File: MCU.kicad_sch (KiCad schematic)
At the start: 44 parts, among them J1 *, J3 *, J4 *, U1 *

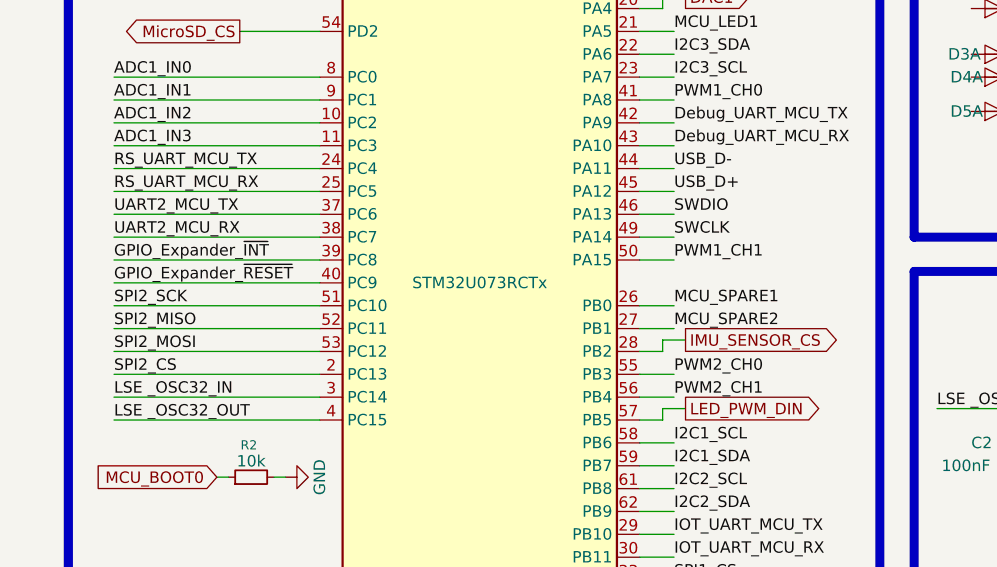
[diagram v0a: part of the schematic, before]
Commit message: [Schematic][Add] MCU Expander Schematic
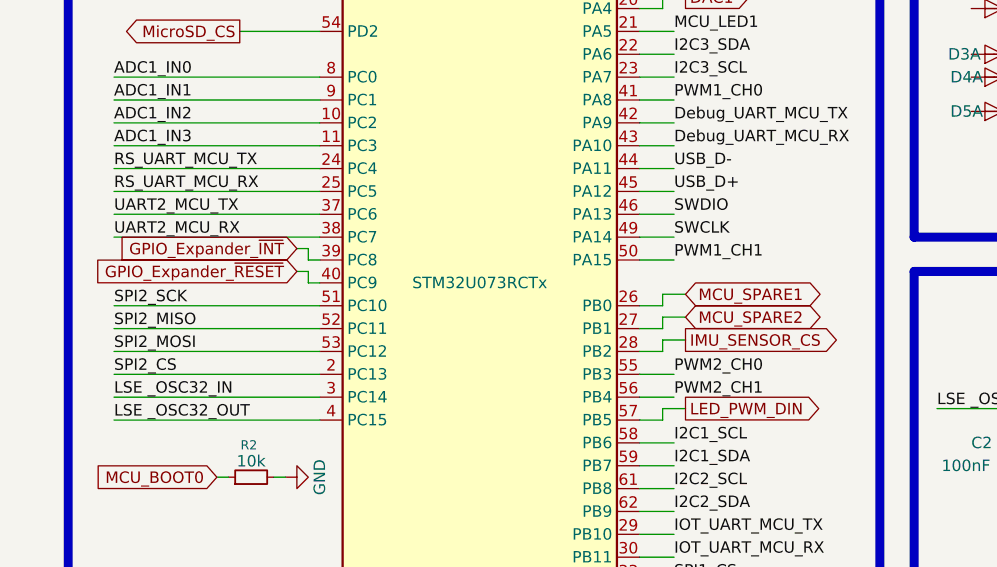
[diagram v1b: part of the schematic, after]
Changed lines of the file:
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@@
 	(wire
 		(pts
+			(xy 82.55 100.33) (xy 82.55 99.06)
+		)
+		(stroke
+			(width 0)
+			(type default)
+		)
+	)
+	(wire
+		(pts
 			(xy 121.92 135.89) (xy 121.92 138.43)
 		)
@@
 	(wire
 		(pts
+			(xy 43.18 95.25) (xy 44.45 95.25)
+		)
+		(stroke
+			(width 0)
+			(type default)
+		)
+	)
+	(wire
+		(pts
 			(xy 250.19 55.88) (xy 269.24 55.88)
 		)
@@
 	(wire
 		(pts
+			(xy 82.55 102.87) (xy 82.55 101.6)
+		)
+		(stroke
+			(width 0)
+			(type default)
+		)
+	)
+	(wire
+		(pts
 			(xy 170.18 50.8) (xy 168.91 50.8)
 		)
@@
 	(wire
 		(pts
+			(xy 82.55 101.6) (xy 85.09 101.6)
+		)
+		(stroke
+			(width 0)
+			(type default)
+		)
+	)
+	(wire
+		(pts
 			(xy 260.35 113.03) (xy 260.35 115.57)
 		)
@@
 	(wire
 		(pts
+			(xy 82.55 99.06) (xy 85.09 99.06)
+		)
+		(stroke
+			(width 0)
+			(type default)
+		)
+	)
+	(wire
+		(pts
+			(xy 41.91 93.98) (xy 43.18 93.98)
+		)
+		(stroke
+			(width 0)
+			(type default)
+		)
+	)
+	(wire
+		(pts
 			(xy 80.01 128.27) (xy 83.82 128.27)
 		)
@@
 	(wire
 		(pts
-			(xy 21.59 97.79) (xy 44.45 97.79)
+			(xy 41.91 96.52) (xy 43.18 96.52)
 		)
 		(stroke
@@
 	(wire
 		(pts
+			(xy 43.18 93.98) (xy 43.18 95.25)
+		)
+		(stroke
+			(width 0)
+			(type default)
+		)
+	)
+	(wire
+		(pts
 			(xy 38.1 170.18) (xy 38.1 171.45)
 		)
@@
 	(wire
 		(pts
+			(xy 43.18 97.79) (xy 44.45 97.79)
+		)
+		(stroke
+			(width 0)
+			(type default)
+		)
+	)
+	(wire
+		(pts
 			(xy 116.84 54.61) (xy 116.84 55.88)
 		)
@@
 	(wire
 		(pts
-			(xy 80.01 102.87) (xy 83.82 102.87)
+			(xy 80.01 102.87) (xy 82.55 102.87)
 		)
 		(stroke
@@
 	(wire
 		(pts
-			(xy 21.59 95.25) (xy 44.45 95.25)
-		)
-		(stroke
-			(width 0)
-			(type default)
-		)
-	)
-	(wire
-		(pts
 			(xy 66.04 168.91) (xy 66.04 170.18)
 		)
@@
 	(wire
 		(pts
-			(xy 80.01 100.33) (xy 83.82 100.33)
+			(xy 80.01 100.33) (xy 82.55 100.33)
 		)
 		(stroke
@@
 	(wire
 		(pts
+			(xy 43.18 96.52) (xy 43.18 97.79)
+		)
+		(stroke
+			(width 0)
+			(type default)
+		)
+	)
+	(wire
+		(pts
 			(xy 152.4 43.18) (xy 152.4 44.45)
 		)
@@
 		)
 	)
-	(label "GPIO_Expander_~{INT}"
-		(at 21.59 95.25 0)
-		(effects
-			(font
-				(size 1.27 1.27)
-			)
-			(justify left bottom)
-		)
-	)
 	(label "Debug_UART_MCU_TX"
 		(at 224.79 46.99 0)
@@
 		)
 	)
-	(label "GPIO_Expander_~{RESET}"
-		(at 21.59 97.79 0)
-		(effects
-			(font
-				(size 1.27 1.27)
-			)
-			(justify left bottom)
-		)
-	)
 	(label "SPI2_MOSI"
 		(at 21.59 105.41 0)
@@
 		)
 	)
-	(label "MCU_SPARE1"
-		(at 83.82 100.33 0)
-		(effects
-			(font
-				(size 1.27 1.27)
-			)
-			(justify left bottom)
-		)
-	)
 	(label "SPI2_SCK"
 		(at 269.24 77.47 180)
@@
 		)
 	)
-	(label "MCU_SPARE2"
-		(at 83.82 102.87 0)
-		(effects
-			(font
-				(size 1.27 1.27)
-			)
-			(justify left bottom)
-		)
-	)
 	(label "I2C3_SCL"
 		(at 83.82 74.93 0)
@@
 		)
 	)
+	(global_label "GPIO_Expander_~{INT}"
+		(shape input)
+		(at 41.91 93.98 180)
+		(fields_autoplaced yes)
+		(effects
+			(font
+				(size 1.27 1.27)
+			)
+			(justify right)
+		)
+		(property "Intersheetrefs" "${INTERSHEET_REFS}"
+			(at 20.9635 93.98 0)
+			(effects
+				(font
+					(size 1.27 1.27)
+				)
+				(justify right)
+				(hide yes)
+			)
+		)
+	)
+	(global_label "MCU_SPARE1"
+		(shape bidirectional)
+		(at 85.09 99.06 0)
+		(fields_autoplaced yes)
+		(effects
+			(font
+				(size 1.27 1.27)
+			)
+			(justify left)
+		)
+		(property "Intersheetrefs" "${INTERSHEET_REFS}"
+			(at 100.2913 99.06 0)
+			(effects
+				(font
+					(size 1.27 1.27)
+				)
+				(justify left)
+				(hide yes)
+			)
+		)
+	)
 	(global_label "MCU_BOOT0"
 		(shape input)
@@
 		)
 	)
+	(global_label "GPIO_Expander_~{RESET}"
+		(shape input)
+		(at 41.91 96.52 180)
+		(fields_autoplaced yes)
+		(effects
+			(font
+				(size 1.27 1.27)
+			)
+			(justify right)
+		)
+		(property "Intersheetrefs" "${INTERSHEET_REFS}"
+			(at 18.1213 96.52 0)
+			(effects
+				(font
+					(size 1.27 1.27)
+				)
+				(justify right)
+				(hide yes)
+			)
+		)
+	)
 	(global_label "DAC1"
 		(shape output)
@@
 			(effects
 				(font
+					(size 1.27 1.27)
+				)
+				(justify left)
+				(hide yes)
+			)
+		)
+	)
+	(global_label "MCU_SPARE2"
+		(shape bidirectional)
+		(at 85.09 101.6 0)
+		(fields_autoplaced yes)
+		(effects
+			(font
+				(size 1.27 1.27)
+			)
+			(justify left)
+		)
+		(property "Intersheetrefs" "${INTERSHEET_REFS}"
+			(at 101.4026 101.6 0)
+			(effects
+				(font
